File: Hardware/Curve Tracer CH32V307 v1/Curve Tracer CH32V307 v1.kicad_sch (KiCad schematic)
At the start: 63 parts, among them J1 To CH32V307, J2 Probes, J3 Power Supply, U1 OPA356xxDBV, U11 ICL7660, U12 LM7805_TO220, U2 AMS1117-3.3, U3 USBLC6-4SC6, U4 OPA356xxDBV, U5 OPA356xxDBV, U6 OPA356xxDBV, U7 MAX393

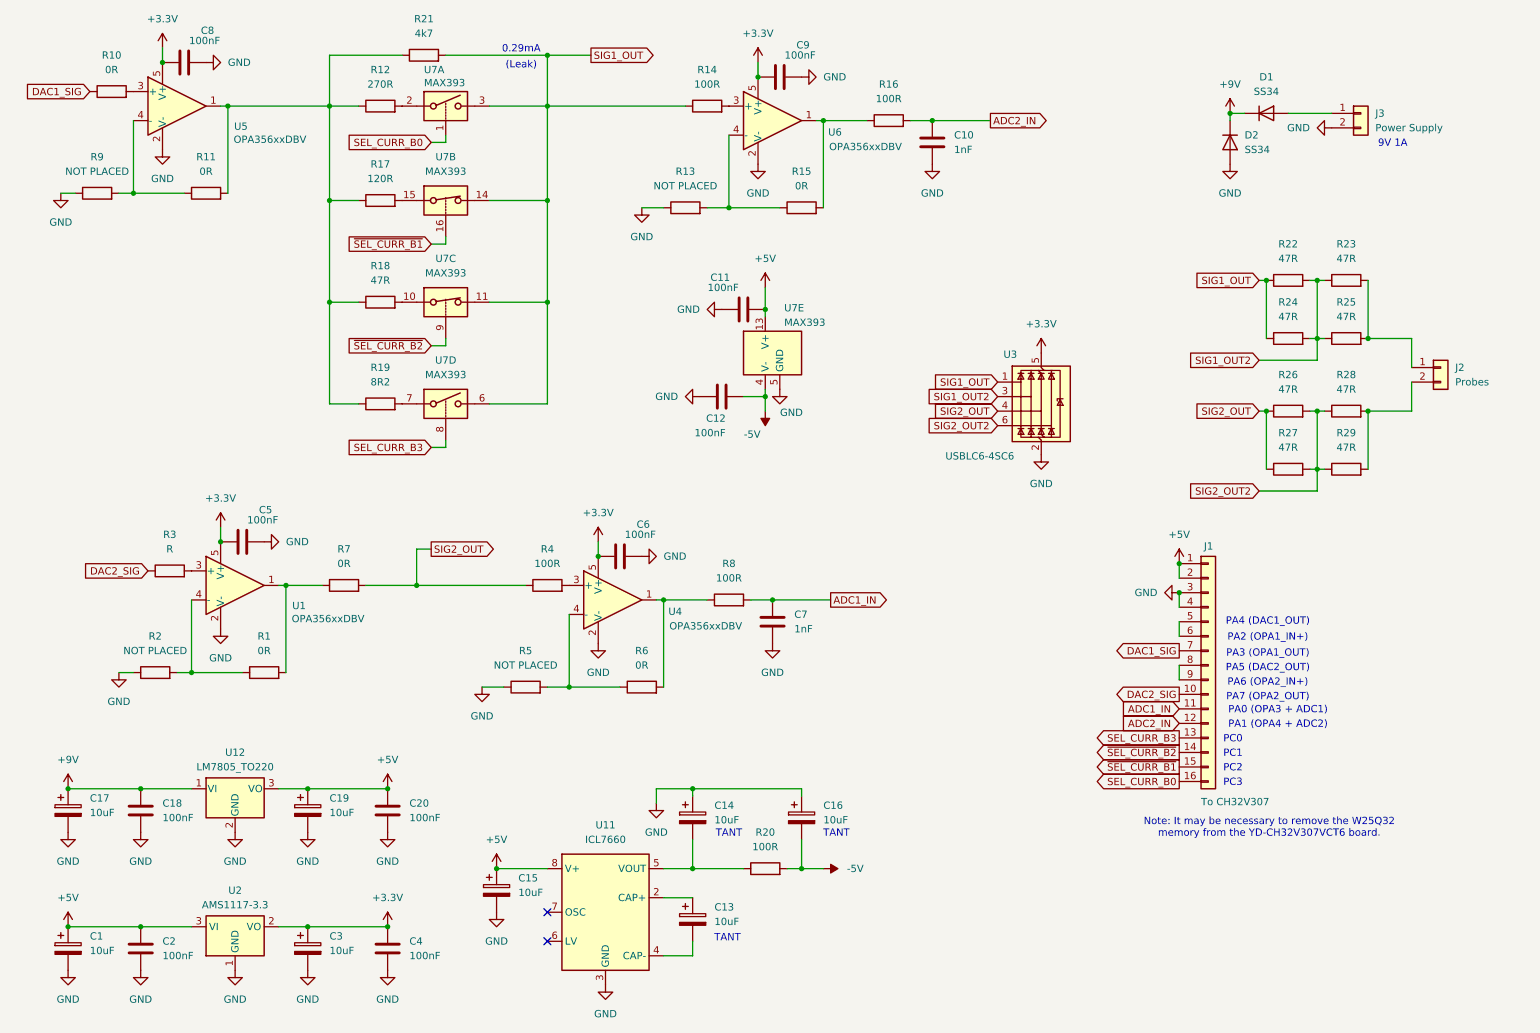
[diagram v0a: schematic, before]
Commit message: Update
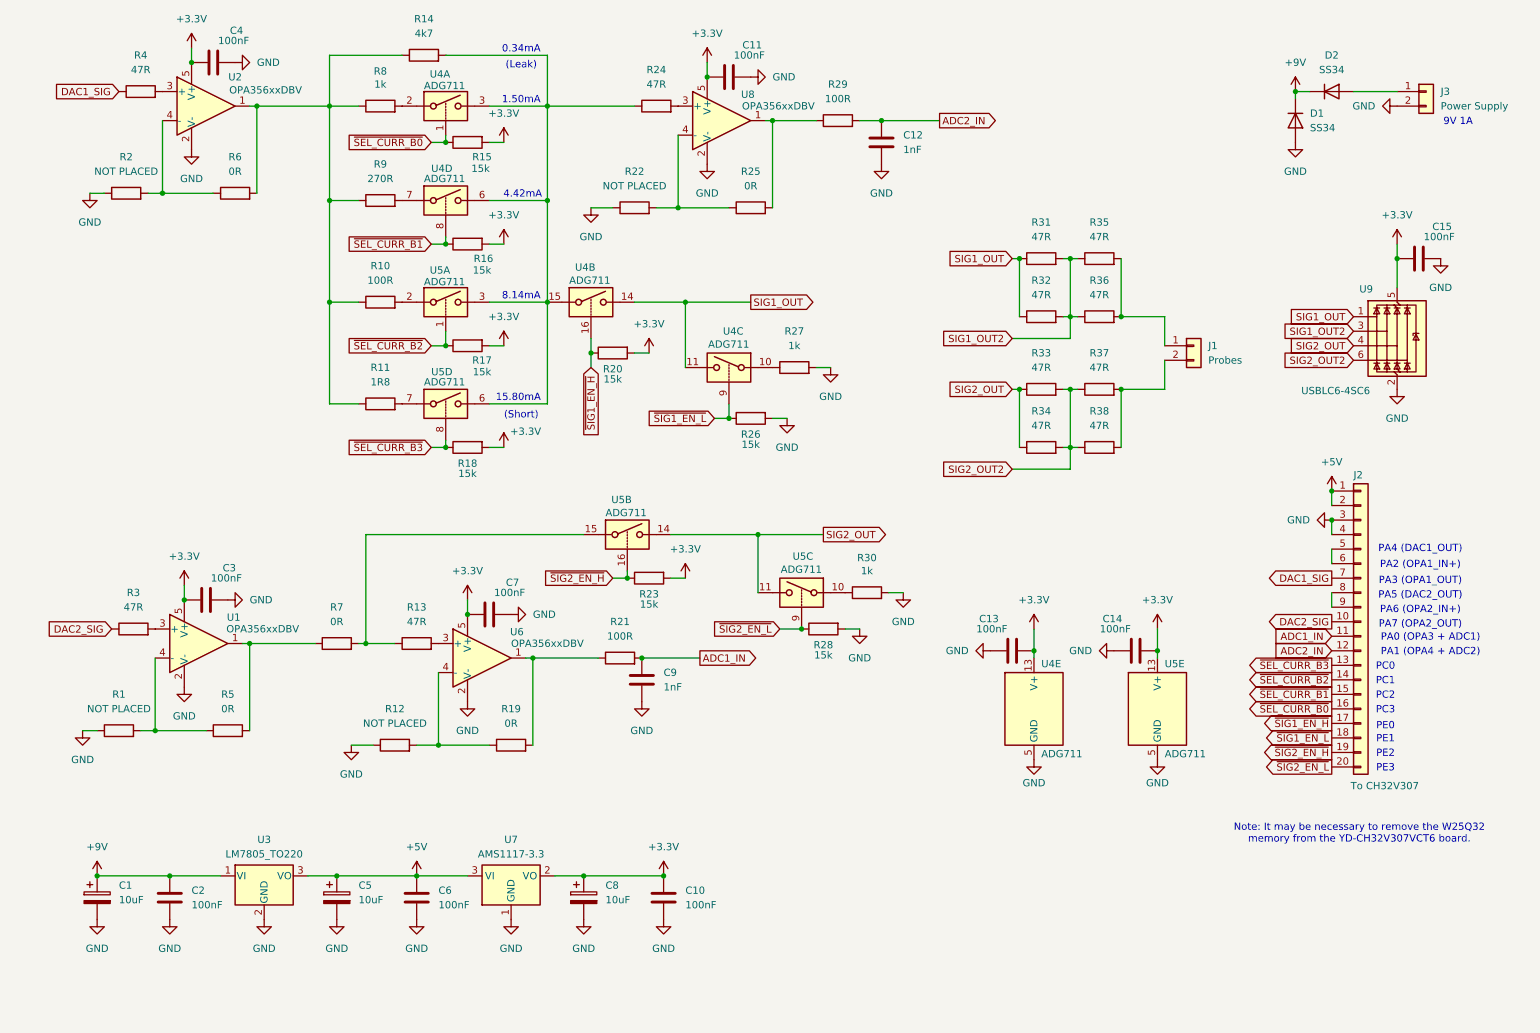
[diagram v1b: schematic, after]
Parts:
- removed C1, C13, C14, C15, C16: 10uF, symbol Device:C_Polarized
- removed C12, C2: 100nF, symbol Device:C
- removed J1: To CH32V307, symbol Connector_Generic:Conn_01x16
- removed U11: ICL7660, symbol Regulator_SwitchedCapacitor:ICL7660
- removed U7: MAX393, Package_SO:SOIC-16_4.55x10.3mm_P1.27mm, symbol MAX393:MAX393
- added C14, C15: 100nF, symbol Device:C
- added J2: To CH32V307, symbol Connector_Generic:Conn_01x20
- added R15, R16, R17, R18, R23, R26, R28: 15k, symbol Device:R
- added R27, R30: 1k, symbol Device:R
- added U4, U5: ADG711, Package_SO:SOIC-16_4.55x10.3mm_P1.27mm, symbol ADG71x:ADG711
- R10: renamed from R18; value 47R -> 100R
- R11: renamed from R19; value 8R2 -> 1R8
- R13: renamed from R4; value 100R -> 47R
- R20: value 100R -> 15k
- R24: renamed from R14; value 100R -> 47R
- R3: value R -> 47R
- R4: renamed from R10; value 0R -> 47R
- R8: renamed from R12; value 270R -> 1k
- R9: renamed from R17; value 120R -> 270R
- renumbered C17 to C1, C4 to C10, C9 to C11, C10 to C12, C11 to C13, C18 to C2, C5 to C3, C8 to C4, C19 to C5, C20 to C6, C6 to C7, C3 to C8, C7 to C9, D2 to D1, D1 to D2, J2 to J1, R2 to R1, R5 to R12, R21 to R14, R6 to R19, R9 to R2, R8 to R21, R13 to R22, R15 to R25, R16 to R29, R22 to R31, R24 to R32, R26 to R33, R27 to R34, R23 to R35, R25 to R36, R28 to R37, R29 to R38, R1 to R5, R11 to R6, U5 to U2, U12 to U3, U4 to U6, U2 to U7, U6 to U8, U3 to U9
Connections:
- net -5V is gone; now on net +3.3V: R20.2
- net +3.3V: now also C13.1, C14.1, C15.1, R15.2, R16.2, R17.2, R18.2, R23.2, U4.13 (V+), U5.13 (V+)
- net +5V: now also J2.1 (Pin_1), J2.2 (Pin_2); no longer C13.1
- net ADC1_IN: now also J2.11 (Pin_11)
- net ADC2_IN: now also J2.12 (Pin_12)
- net DAC1_SIG: now also J2.7 (Pin_7)
- net DAC2_SIG: now also J2.10 (Pin_10)
- net GND: now also C14.2, C15.2, J2.3 (Pin_3), J2.4 (Pin_4), R26.2, R27.2, R28.2, R30.2, U4.5 (GND), U5.5 (GND)
- net SIG1_OUT: now also U4.11, U4.14; no longer R14.2, R24.1
- net SIG2_OUT: now also U5.11, U5.14; no longer R13.1, R7.2
- net ~{SEL_CURR_B1}: now also J2.15 (Pin_15), R16.1, U4.8
- net ~{SEL_CURR_B2}: now also J2.14 (Pin_14), R17.1, U5.1
- net at R11.2: now also U5.7
- net at R8.2: now also U4.2
- net at R9.2: now also U4.7
- net at R10.2: now also U5.2
- net ~{SIG1_EN_H}: now reaches R20.1
- net ~{SIG1_EN_H}: now also J2.17 (Pin_17), U4.16
- new net: R14.2, R24.1, U4.15, U4.3, U4.6, U5.3, U5.6
- new net: R13.1, R7.2, U5.15
- new net: R30.1, U5.10
- new net: R27.1, U4.10
- new net: J2.5 (Pin_5), J2.6 (Pin_6)
- new net: J2.8 (Pin_8), J2.9 (Pin_9)
- new net ~{SEL_CURR_B0}: J2.16 (Pin_16), R15.1, U4.1
- new net ~{SEL_CURR_B3}: J2.13 (Pin_13), R18.1, U5.8
- new net ~{SIG1_EN_L}: J2.18 (Pin_18), R26.1, U4.9
- new net ~{SIG2_EN_H}: J2.19 (Pin_19), R23.1, U5.16
- new net ~{SIG2_EN_L}: J2.20 (Pin_20), R28.1, U5.9
- no-connect marks 2 -> 0
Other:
- note added: "(Short)"
- note added: "0.34mA"
- note added: "1.50mA"
- note added: "15.80mA"
- note added: "4.42mA"
- note added: "8.14mA"
- note added: "PE0"
- note added: "PE1"
- note added: "PE2"
- note added: "PE3"
- note removed: "0.29mA"
- note removed: "TANT"
- moved on the sheet: C1, C10, C11, C12, C13, C2, C3, C4, C5, C6, C7, C8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
